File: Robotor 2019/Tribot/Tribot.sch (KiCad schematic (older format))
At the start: 73 parts, among them J1 Conn_01x03_Male, J2 Conn_01x04_Female, J3 USB_B_Mini, J4 Conn_01x04_Female, J5 Conn_01x04_Female, J6 Conn_01x04_Female, J7 Conn_01x03_Female, J8 Conn_01x03_Female, M1 Motor_DC, M2 Motor_DC, U1 AMS1117-3V3, U2 AMS1117-3V3, U3 AMS1117-5.0, U4 STM32F103C8Tx, U5 ITR8307, U6 L298P, U7 ITR8307, U8 ITR8307, U9 ITR8307, Y1 32.768Khz, Y2 8Mhz

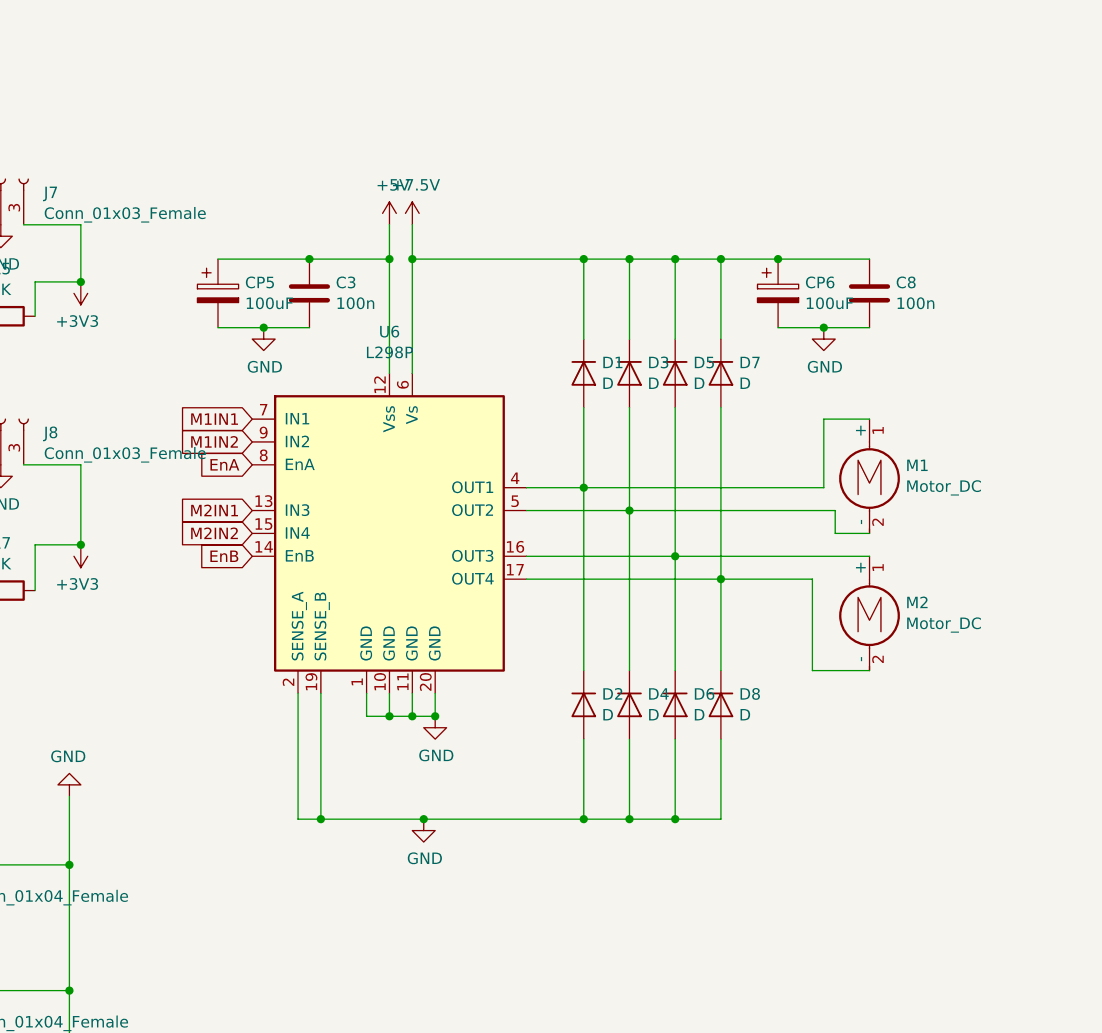
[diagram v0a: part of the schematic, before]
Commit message: The PCB for Tribot up to the point we realised we need a 2nd floor.
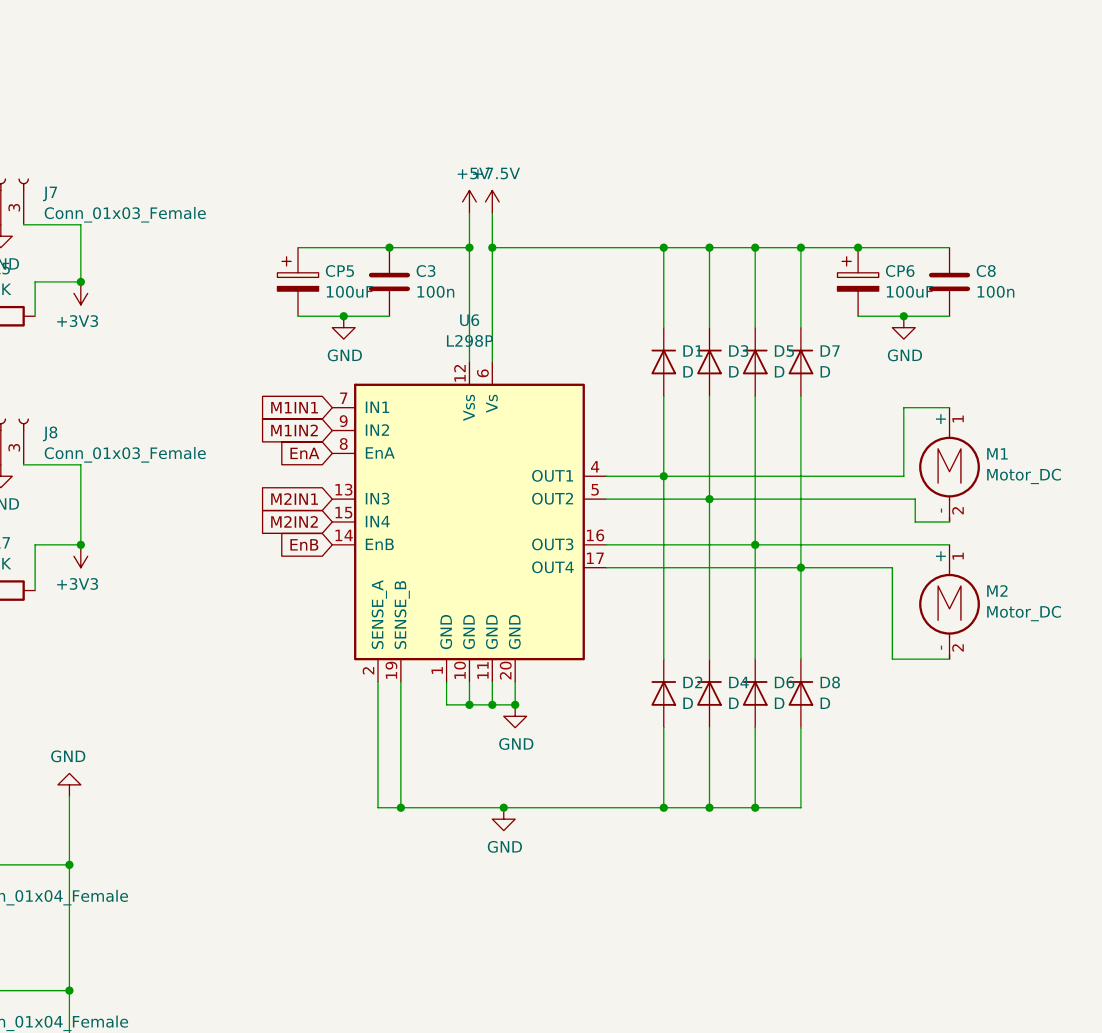
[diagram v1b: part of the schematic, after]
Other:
- moved on the sheet: C3, C8, CP5, CP6, D1, D2, D3, D4, D5, D6, D7, D8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
